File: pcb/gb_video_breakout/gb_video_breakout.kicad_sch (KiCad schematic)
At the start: 12 parts, among them J1 Conn_01x05, Q1 MMBF170, Q2 MMBF170, U1 SN74LVC1G17QDCKRQ1, U2 SN74LVC1G17QDCKRQ1

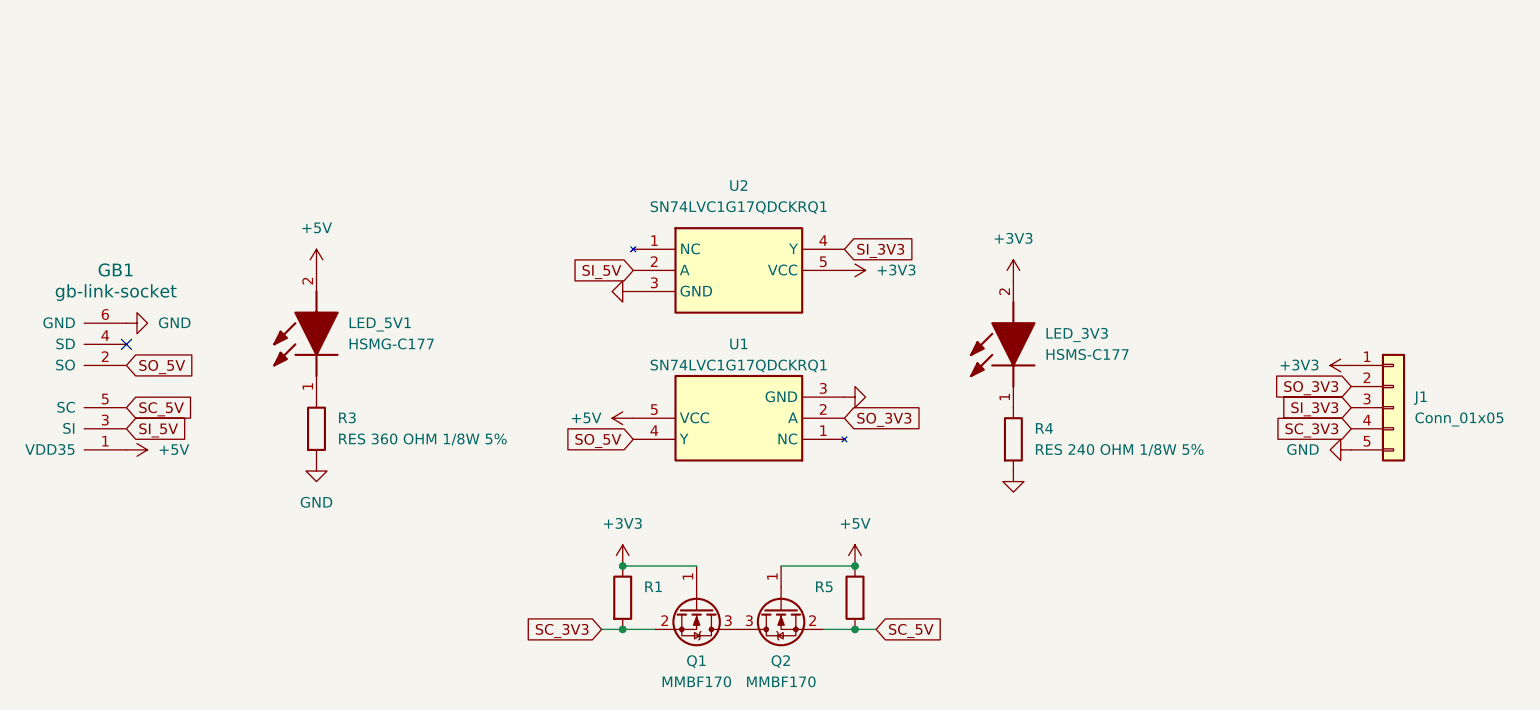
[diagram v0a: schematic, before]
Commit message: V0.5
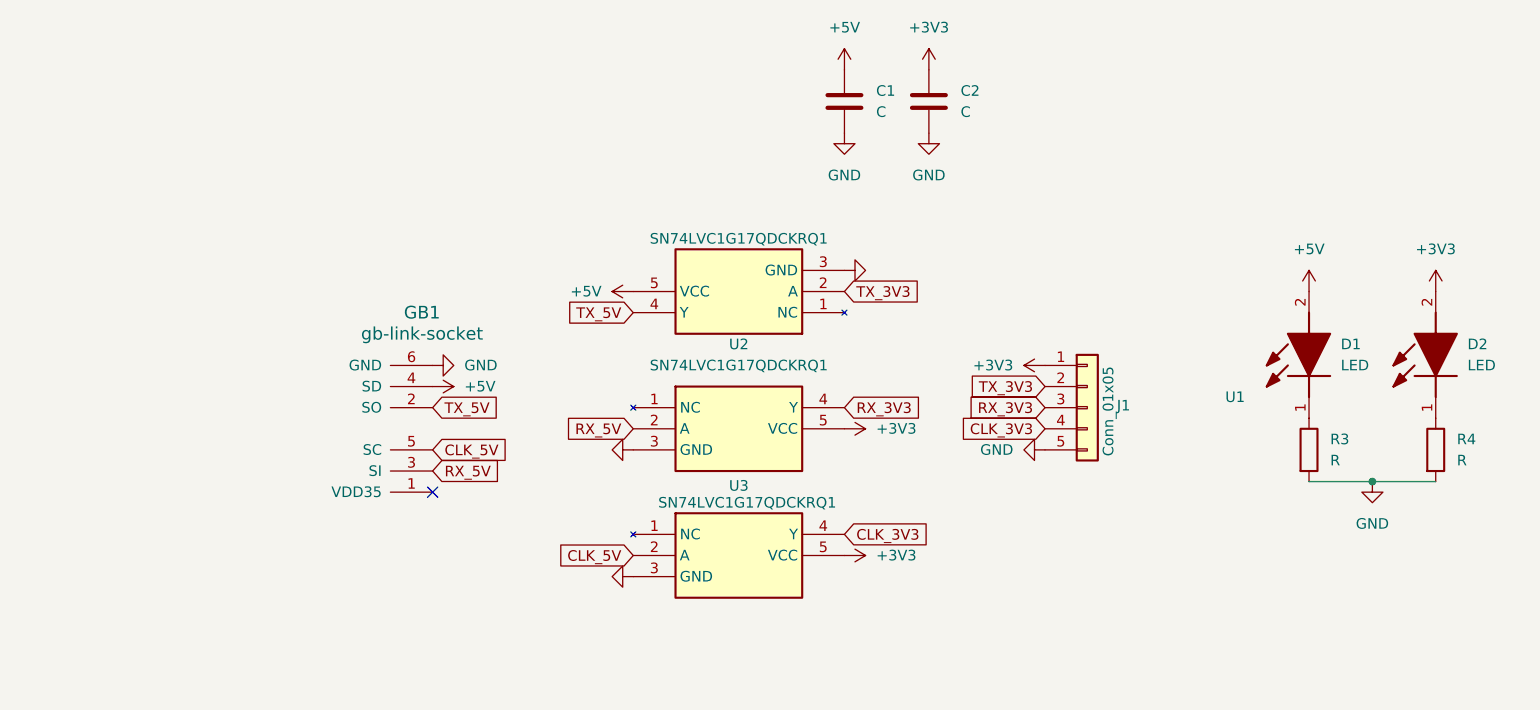
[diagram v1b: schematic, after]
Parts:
- removed Q1, Q2: MMBF170, Package_TO_SOT_SMD:SOT-23, symbol Transistor_FET:BS170F
- removed R1, R5: RES 1K OHM 1%, Resistor_SMD:R_1206_3216Metric, symbol Device:R
- added C1, C2: C, Capacitor_SMD:C_0805_2012Metric, symbol Device:C
- added U3: SN74LVC1G17QDCKRQ1, SOT65P210X110-5N, symbol SN74LVC1G17QDCKRQ1:SN74LVC1G17QDCKRQ1
- D1: renamed from LED_5V1; value HSMG-C177 -> LED; footprint LED_SMD:LED_1206_3216Metric -> LED_SMD:LED_0805_2012Metric
- D2: renamed from LED_3V3; value HSMS-C177 -> LED; footprint LED_SMD:LED_1206_3216Metric -> LED_SMD:LED_0805_2012Metric
- R3: value RES 360 OHM 1/8W 5% -> R; footprint Resistor_SMD:R_1206_3216Metric -> Resistor_SMD:R_0805_2012Metric
- R4: value RES 240 OHM 1/8W 5% -> R; footprint Resistor_SMD:R_1206_3216Metric -> Resistor_SMD:R_0805_2012Metric
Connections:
- net +3V3: now also C2.1, U3.5 (VCC)
- net +5V: now also GB1.4 (SD), C1.1; no longer GB1.1 (VDD35)
- net GND: now also C1.2, C2.2, U3.3 (GND)
- net SC_3V3 renamed CLK_3V3
- net CLK_3V3: now also U3.4 (Y)
- net SC_5V renamed CLK_5V
- net CLK_5V: now also U3.2 (A)
- net SI_3V3 renamed RX_3V3
- net SI_5V renamed RX_5V
- net SO_3V3 renamed TX_3V3
- net SO_5V renamed TX_5V
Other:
- moved on the sheet: D1, D2, GB1, J1, R3, R4, U1, U2
